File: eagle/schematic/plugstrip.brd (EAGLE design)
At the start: 279.4 x 293.4 mm, 14 parts, among them J1 213598-2, U1 Hall Effect, U2 Current ADC, U3 Voltage ADC

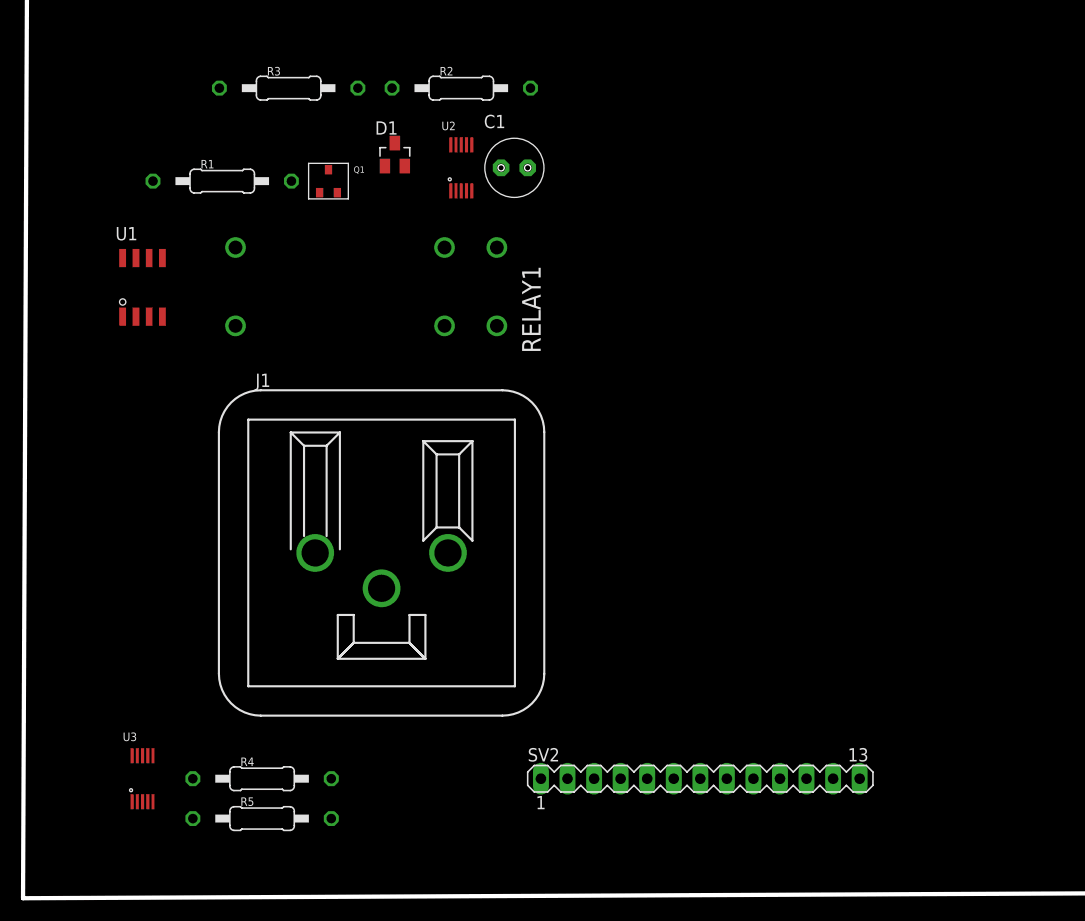
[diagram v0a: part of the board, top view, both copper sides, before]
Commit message: update
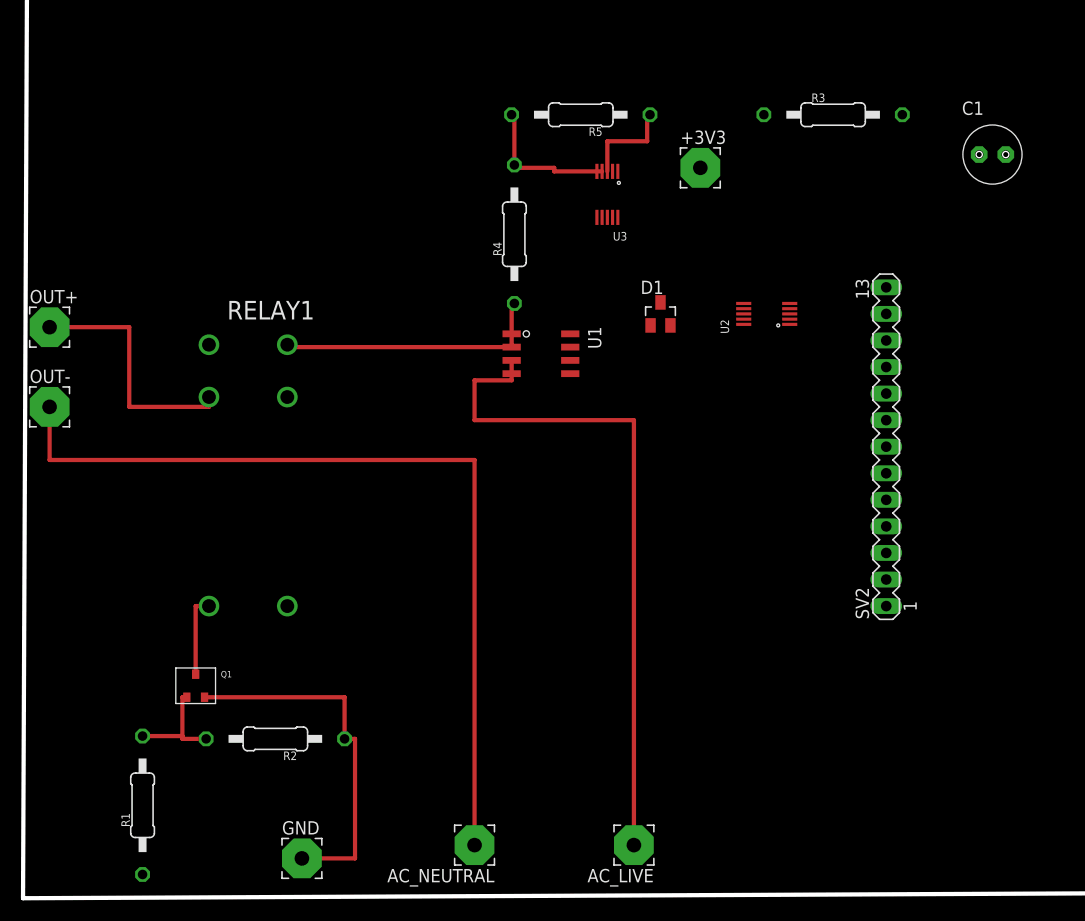
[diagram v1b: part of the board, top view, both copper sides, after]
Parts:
- removed J1: 213598-2, con-amp:213598-2
- added +3V3, AC_LIVE, AC_NEUTRAL, GND, OUT+, OUT-: (no value), wirepad:3,81/1,4
- moved R5 73.9 mm to (52.1, 73.7), turned to 180 degrees
- moved U3 71.4 mm to (54.6, 66.0), turned to 180 degrees
- moved R2 64.7 mm to (22.9, 14.0), turned to 180 degrees
- moved R1 60.2 mm to (10.2, 7.62), turned to 90 degrees
- moved R4 57.4 mm to (45.7, 62.2), turned to 90 degrees
- moved R3 52.1 mm to (76.2, 73.7)
- moved Q1 49.9 mm to (15.2, 19.1)
- moved C1 45.7 mm to (91.4, 69.8)
- moved U1 38.6 mm to (48.3, 50.8), turned to 270 degrees
- moved SV2 36.4 mm to (81.3, 41.9), turned to 90 degrees
- moved U2 32.4 mm to (69.8, 54.6), turned to 90 degrees
- moved D1 29.6 mm to (59.7, 54.6)
- moved RELAY1 19.4 mm to (21.6, 39.4), turned to 90 degrees
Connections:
- new net N$4: +3V3.1, U3.P$8
- net +3V3: no longer U3.P$8
- net AC_LIVE: now also AC_LIVE.1
- net AC_NEUTRAL: now also AC_NEUTRAL.1, OUT-.1; no longer RELAY1.IN2
- net GND: now also GND.1; no longer U3.P$5
- net N$1: now also OUT+.1, RELAY1.IN1; no longer J1.3, RELAY1.OUT1
- net N$2: now also RELAY1.OUT1; no longer J1.2, RELAY1.IN1
- net N$31: now also U3.P$5
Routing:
- net AC_NEUTRAL: track 0.00 -> 82.5 mm
- net AC_LIVE: track 0.00 -> 65.1 mm
- net GND: track 0.00 -> 44.4 mm
- net N$3: track 0.00 -> 26.3 mm
- net N$1: track 0.00 -> 23.8 mm
- net N$31: track 0.00 -> 14.1 mm
- net N$6: track 0.00 -> 10.5 mm
- net N$5: track 0.00 -> 7.79 mm
